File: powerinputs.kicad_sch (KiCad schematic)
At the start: 6 parts, among them J10 Conn_02x02_Odd_Even, J9 Barrel_Jack

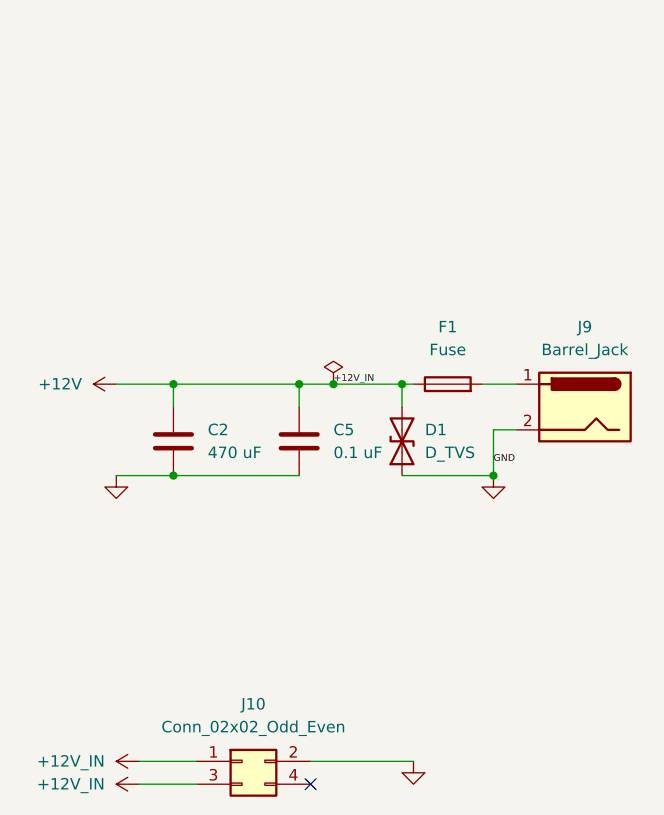
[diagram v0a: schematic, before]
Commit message: only da inductor
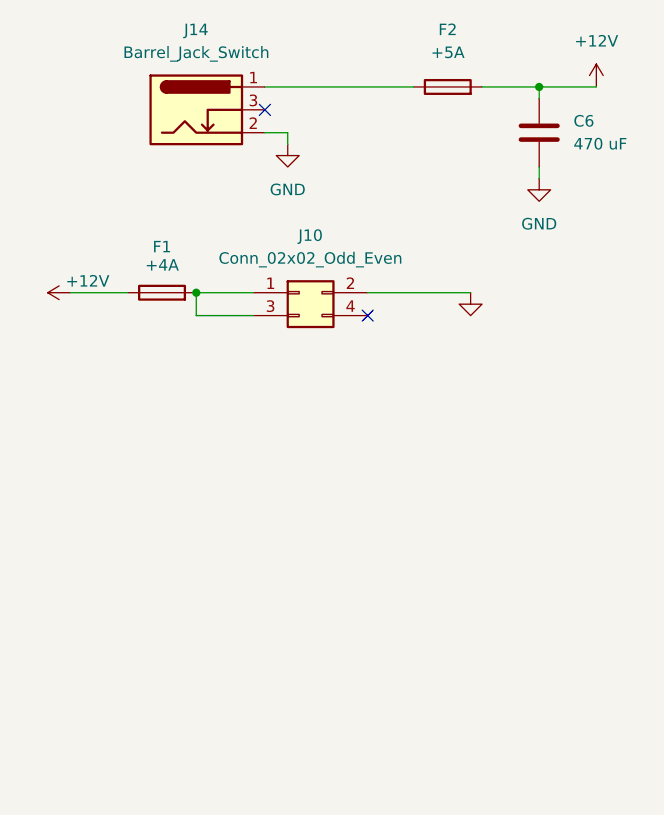
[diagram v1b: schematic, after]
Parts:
- removed C2: 470 uF, symbol Device:C
- removed C5: 0.1 uF, symbol Device:C
- removed D1: D_TVS, symbol Device:D_TVS
- removed J9: Barrel_Jack, symbol Connector:Barrel_Jack
- added C6: 470 uF, Capacitor_SMD:C_0603_1608Metric_Pad1.08x0.95mm_HandSolder, symbol Device:C
- added F2: +5A, Fuse:Fuseholder_Blade_Mini_Keystone_3568, symbol Device:Fuse
- added J14: Barrel_Jack_Switch, KiCad:694108301002, symbol Connector:Barrel_Jack_Switch
- F1: value Fuse -> +4A; footprint (none) -> Fuse:Fuseholder_Blade_Mini_Keystone_3568
- J10: footprint (none) -> Connector_Molex:Molex_Nano-Fit_105310-xx04_2x02_P2.50mm_Vertical
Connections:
- net +12V: now also C6.1, F2.2; no longer J10.1 (Pin_1), J10.3 (Pin_3)
- net GND: now also C6.2, J14.2
- net at F1.2: now also J10.1 (Pin_1), J10.3 (Pin_3)
- new net: F2.1, J14.1
- no-connect marks 1 -> 2
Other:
- moved on the sheet: J10
